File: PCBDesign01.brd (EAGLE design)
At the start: 100 x 80 mm, 14 parts, among them IC1 TESEO-LIV3R, U2 VX7805-500

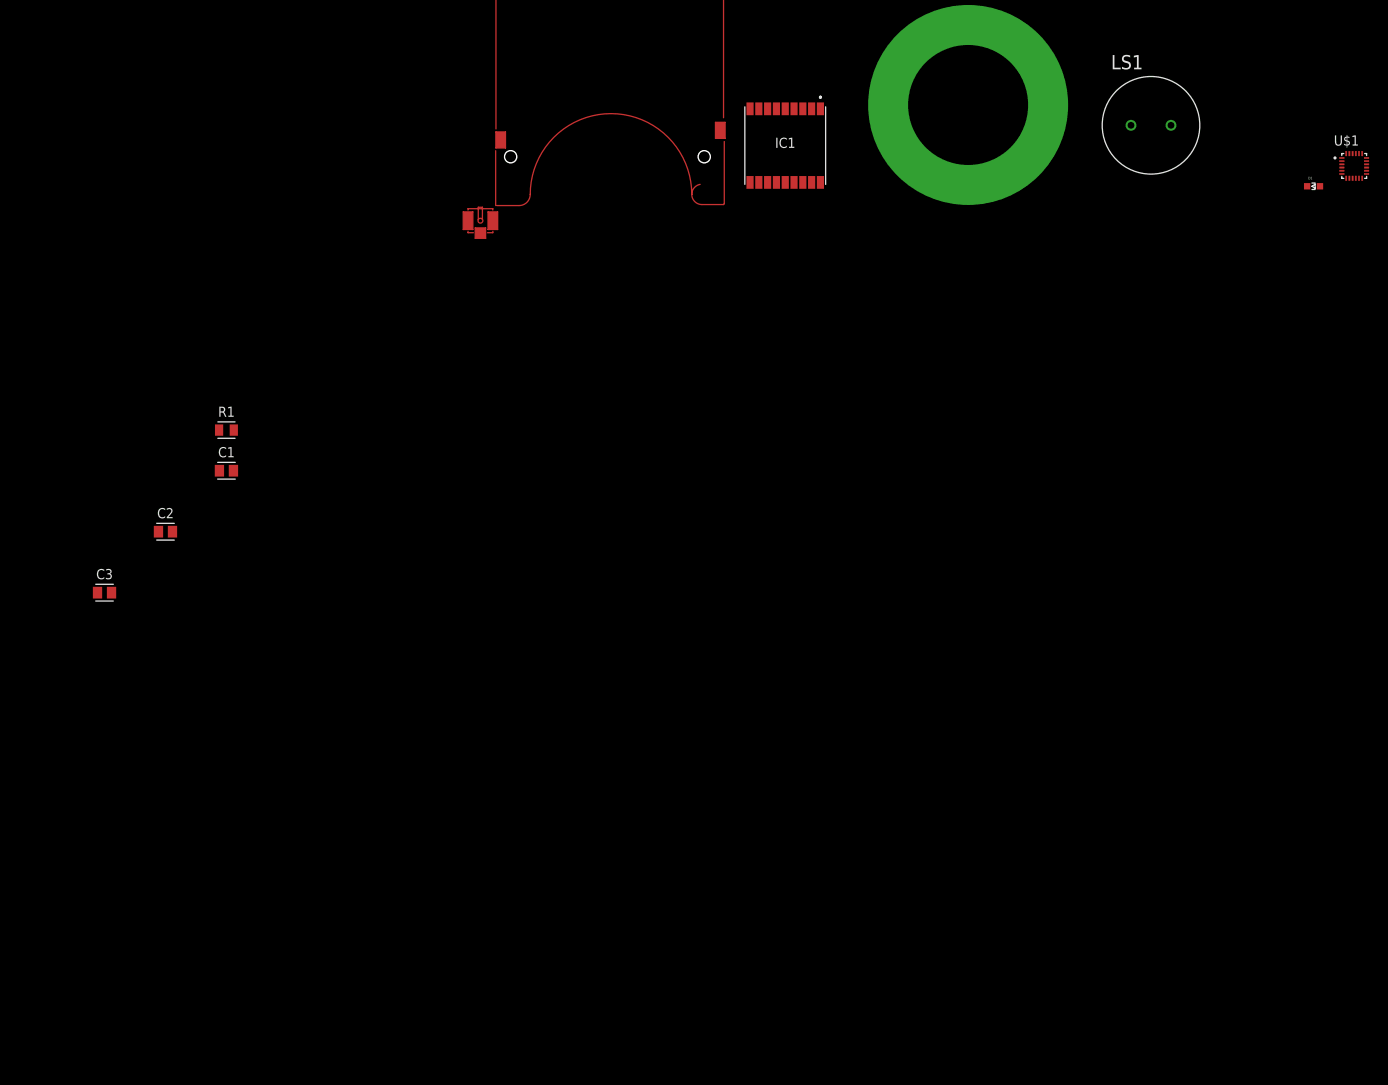
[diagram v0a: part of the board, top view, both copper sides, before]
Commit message: more stuff
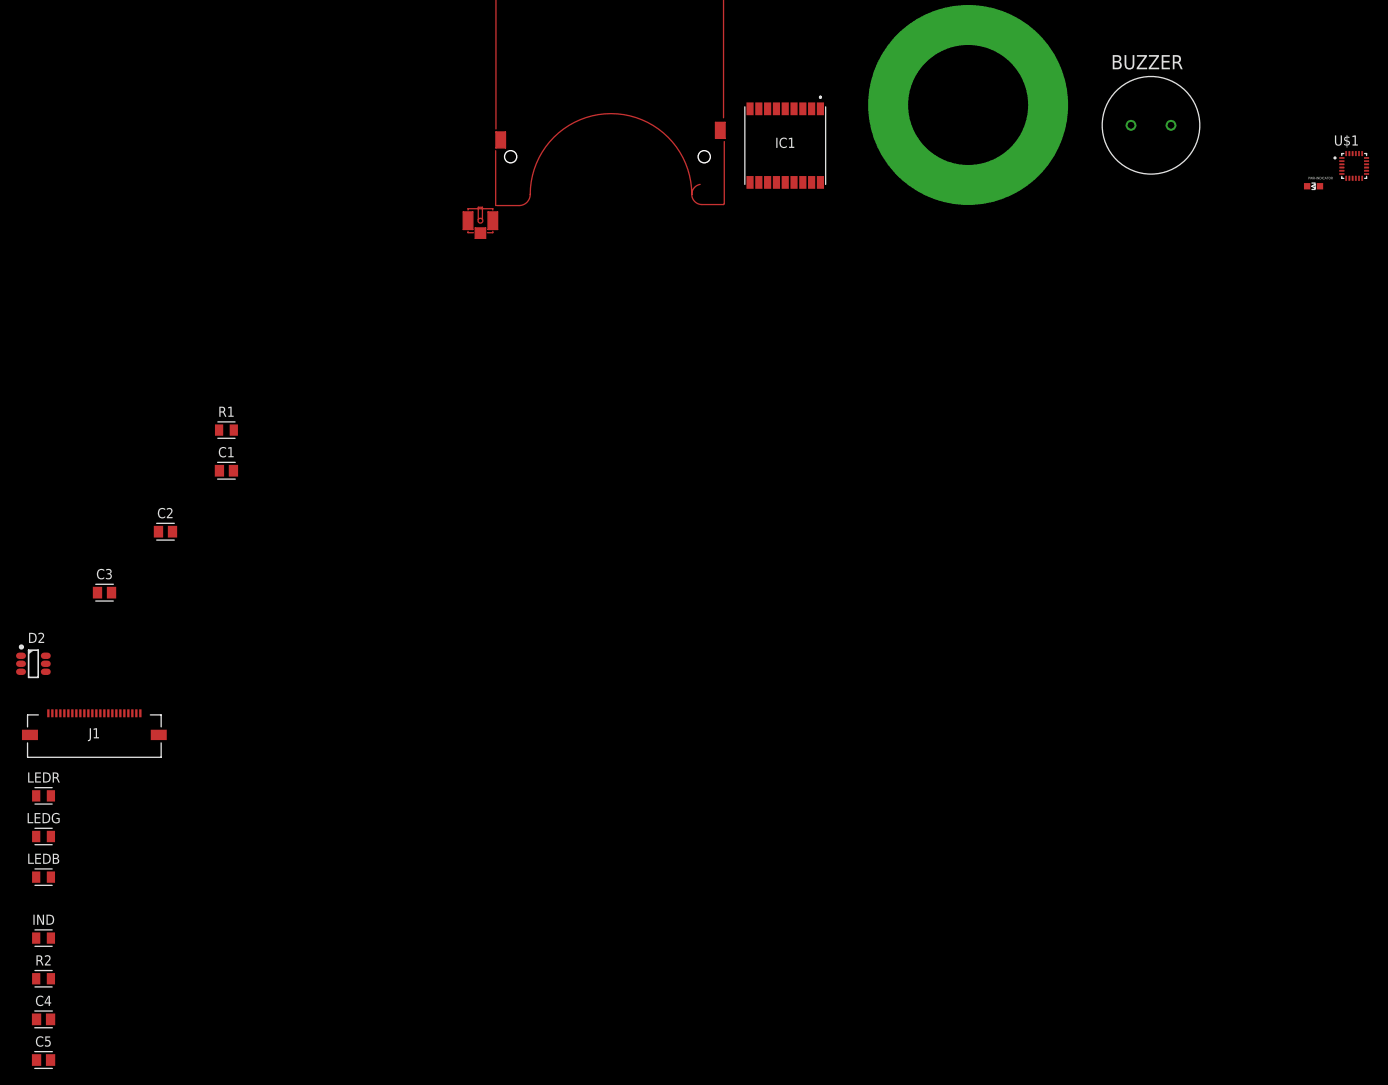
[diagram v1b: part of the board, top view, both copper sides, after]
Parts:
- added C4, C5: (no value), Capacitor:CAPC2012X110
- added D2: CLX6F-FKC-CKNNQDGBB7A363, CLX6F-FKC-CKNNQDGBB7A363:SOJ100P350X290-6N
- added IND, LEDB, LEDG, LEDR, R2: (no value), Resistor:RESC2012X65
- added J1: 5051102491, 5051102491:5051102491
- C1, C2, C3: value C_CHIP-0805(2012-METRIC) -> (none)
- renumbered D1 to PWR-INDICATOR, LS1 to BUZZER
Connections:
- new net N$1: D2.3, LEDR.1
- new net N$2: D2.2, LEDG.1
- new net N$4: D2.1, LEDB.1
- new net N$6: IND.1, PWR-INDICATOR.1
- new net N$7: J1.17, R2.1
- new net N$8: C5.1, J1.14
- new net N$9: C4.1, J1.8
- net GND: now also BUZZER.2, C4.2, C5.2, IND.2, J1.10, J1.23, J1.25, J1.26, LEDB.2, LEDG.2, LEDR.2, R2.2
